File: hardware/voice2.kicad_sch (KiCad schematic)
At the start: 30 parts, among them IC1 LM13700, U12 MCP4922-E/P, U9 SSI2144

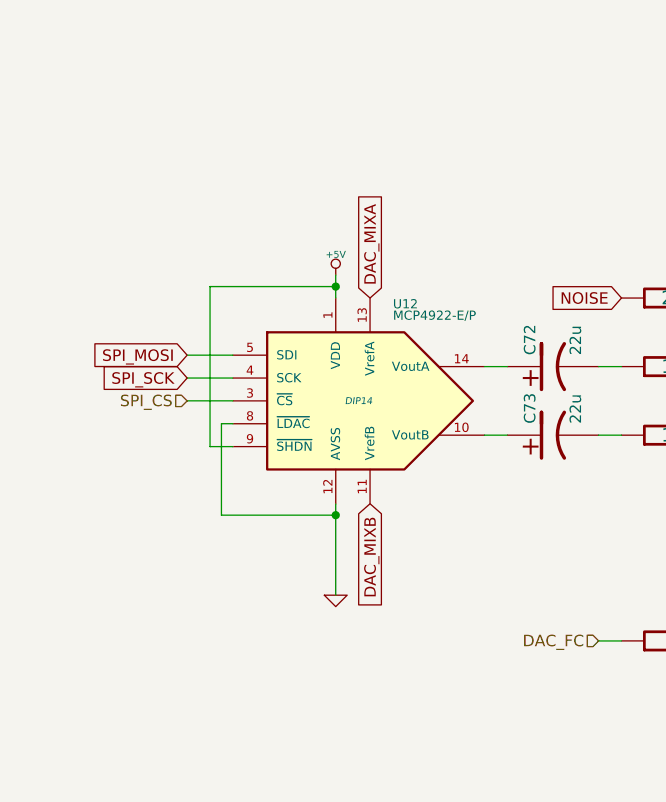
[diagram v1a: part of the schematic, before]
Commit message: hardware: sch small changes -- footprints assigned
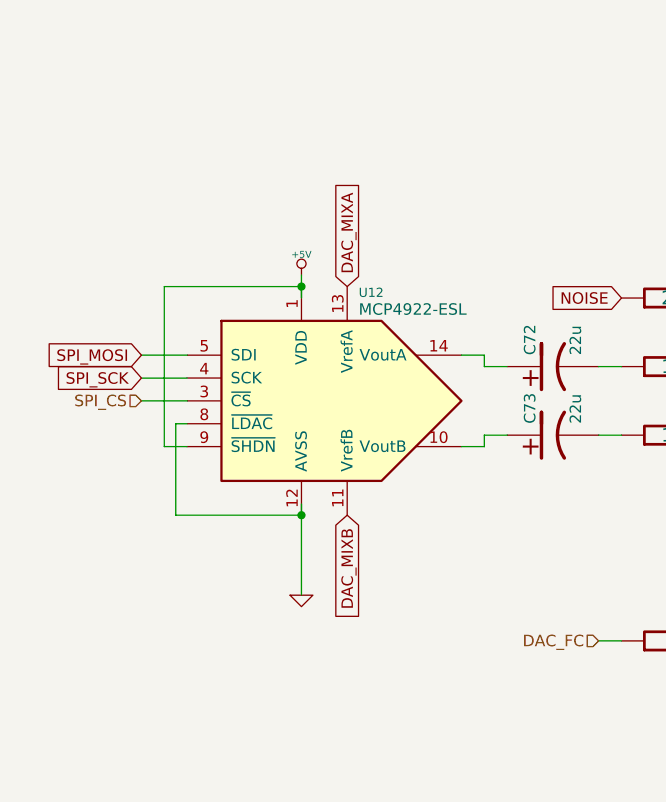
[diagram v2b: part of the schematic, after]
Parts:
- C72, C73, C79: footprint ~ -> Capacitor_Tantalum_SMD:CP_EIA-3216-18_Kemet-A
- C74, C80: footprint ~ -> Capacitor_SMD:C_0805_2012Metric
- C75, C76, C77: footprint ~ -> Capacitor_SMD:C_1206_3216Metric
- C78: footprint ~ -> Capacitor_SMD:C_0603_1608Metric
- C81: footprint ~ -> Capacitor_Tantalum_SMD:CP_EIA-3528-21_Kemet-B
- IC1: footprint (none) -> Package_SO:SO-16_3.9x9.9mm_P1.27mm
- R86, R87, R89, R90, R91, R92, R93, R94, R95, R96, R97, R98, R99: footprint ~ -> Resistor_SMD:R_0805_2012Metric
- U12: value MCP4922-E/P -> MCP4922-ESL; footprint DIP14 -> Package_SO:SO-14_3.9x8.65mm_P1.27mm; symbol overcycler2-rescue:MCP4922-E/P -> Analog_DAC:MCP4922-ESL
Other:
- moved on the sheet: U12
